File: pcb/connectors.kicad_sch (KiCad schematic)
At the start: 7 parts, among them J1 USB_C_Receptacle_USB2.0, J5 Conn_01x04, U6 USBLC6-2SC6

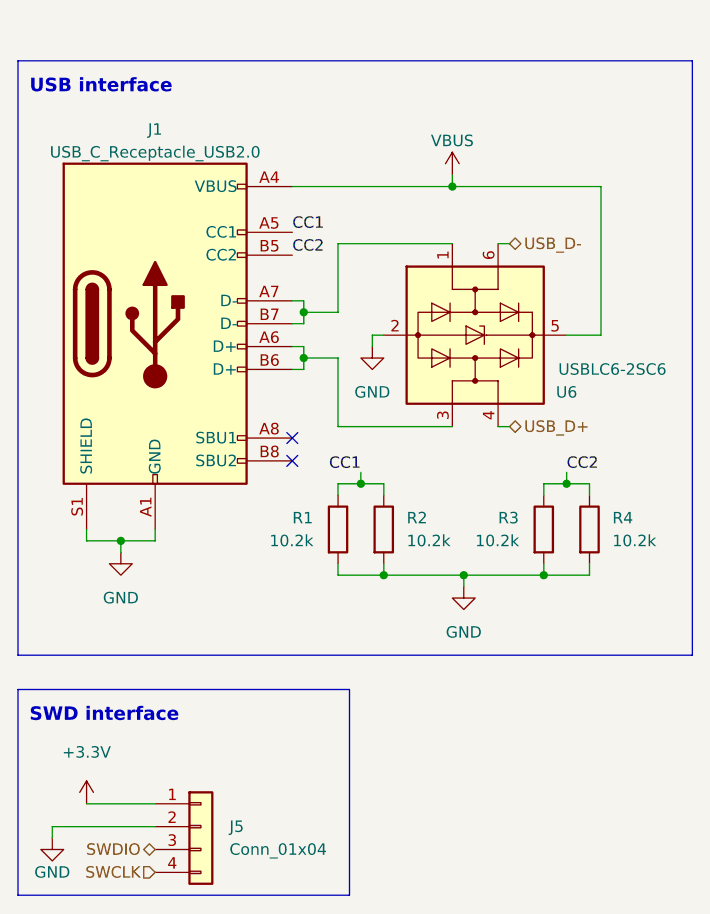
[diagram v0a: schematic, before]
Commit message: Schematic done, starting PCB design
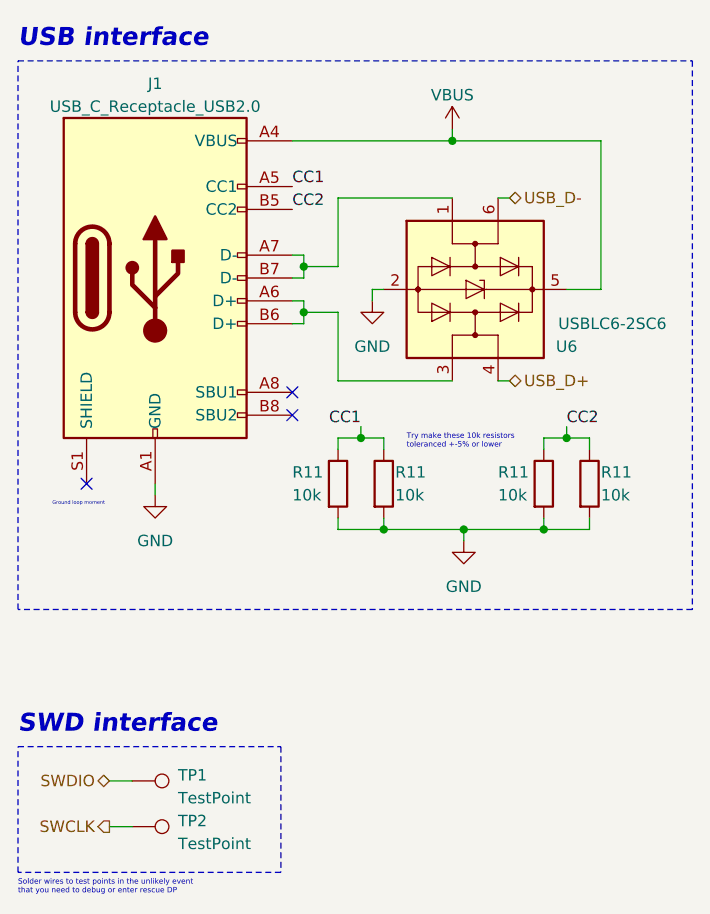
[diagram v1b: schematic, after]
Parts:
- removed J5: Conn_01x04, Connector_PinSocket_2.54mm:PinSocket_1x04_P2.54mm_Horizontal, symbol Connector_Generic:Conn_01x04
- removed R1, R2, R3, R4: 10.2k, Resistor_SMD:R_0603_1608Metric, symbol Device:R
- added R11 (x4): 10k, Resistor_SMD:R_0603_1608Metric_Pad0.98x0.95mm_HandSolder, symbol Device:R
- added TP1, TP2: TestPoint, TestPoint:TestPoint_Pad_D2.0mm, symbol Connector:TestPoint
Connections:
- net CC1: now also R11.1, R11.1
- net CC2: now also R11.1, R11.1
- net GND: now also R11.2, R11.2, R11.2, R11.2; no longer J1.S1 (SHIELD)
- net SWCLK: now also TP2.1
- net SWDIO: now also TP1.1
- no-connect marks 2 -> 3
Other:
- note added: "Ground loop moment"
- note added: "Solder wires to test points in the unlikely event that you need to debug or enter rescue DP"
- note added: "Try make these 10k resistors toleranced +-5% or lower"
- moved on the sheet: J1, U6
